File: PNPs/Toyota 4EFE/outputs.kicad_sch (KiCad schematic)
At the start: 9 parts, among them Q2 SSM3K357R, Q3 SSM3K357R, U9 VNLD5090

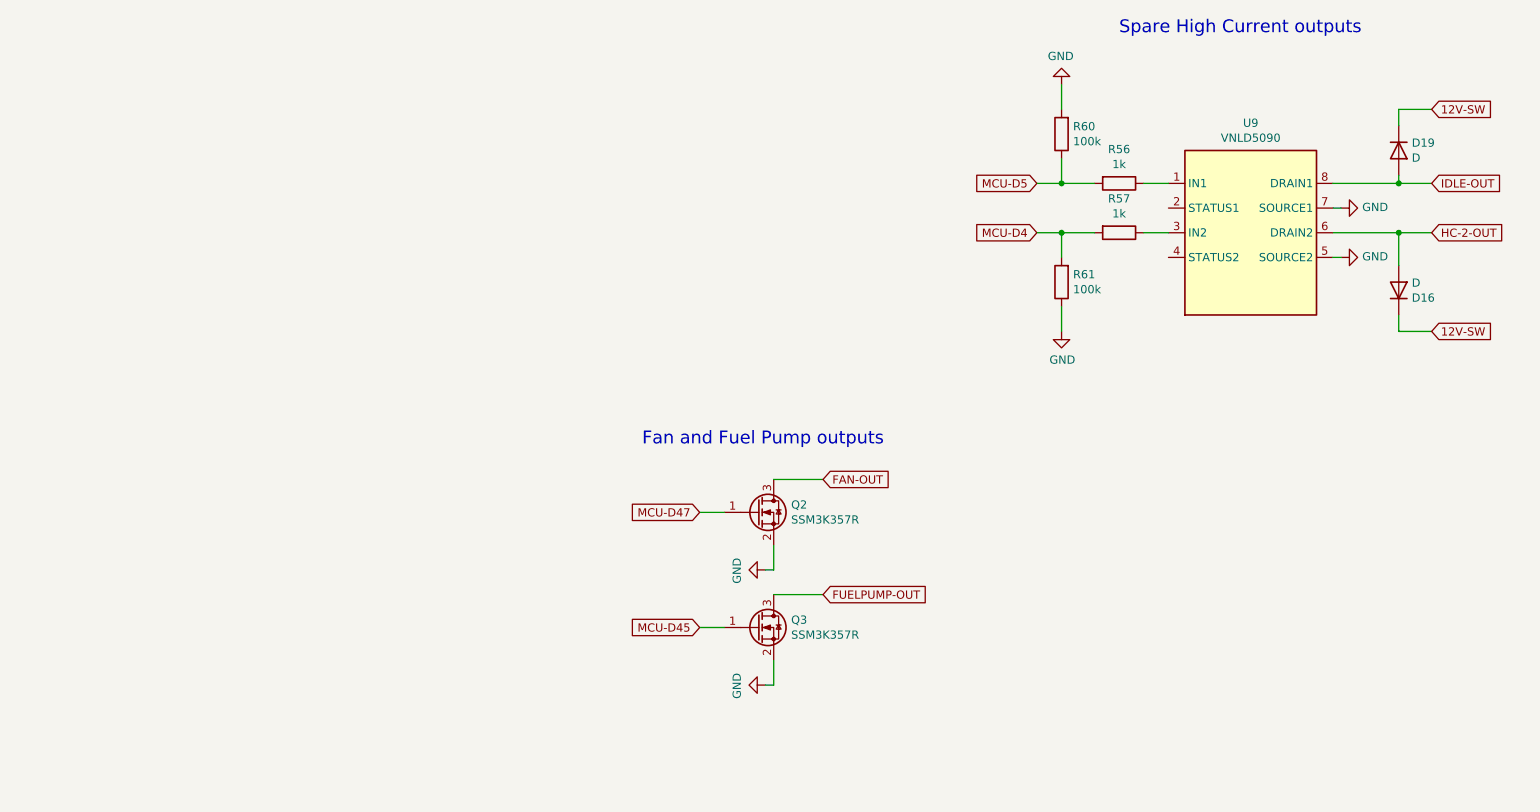
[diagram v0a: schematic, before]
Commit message: Board layout done
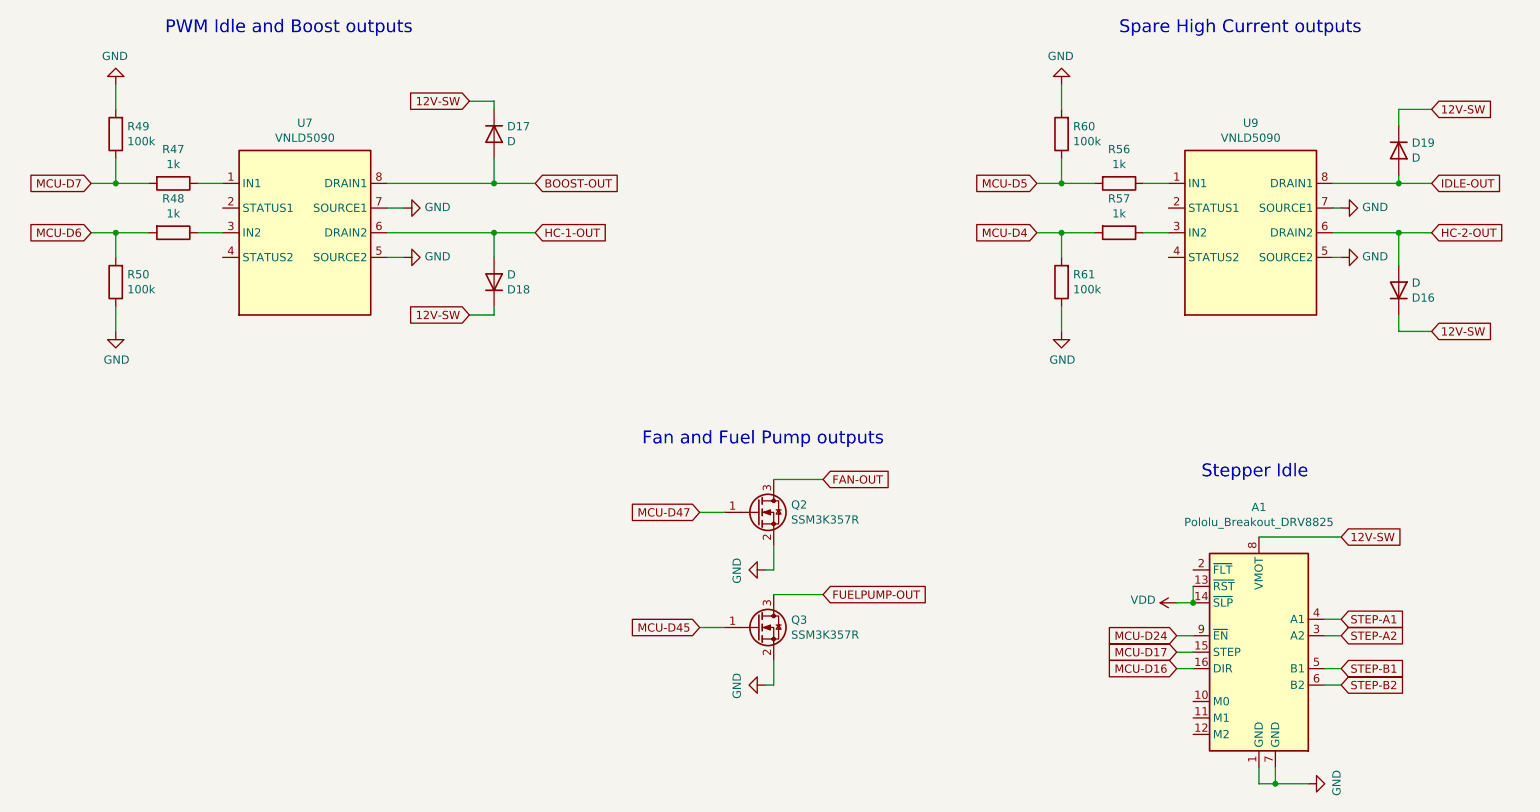
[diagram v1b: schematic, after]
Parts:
- added A1: Pololu_Breakout_DRV8825, Module:Pololu_Breakout-16_15.2x20.3mm, symbol Driver_Motor:Pololu_Breakout_DRV8825
- added D17, D18: D, Diode_SMD:D_SOD-123F, symbol Device:D
- added R47, R48: 1k, Resistor_SMD:R_0805_2012Metric, symbol Device:R
- added R49, R50: 100k, Resistor_SMD:R_0805_2012Metric, symbol Device:R
- added U7: VNLD5090, Package_SO:SOIC-8_3.9x4.9mm_P1.27mm, symbol v0.4.4c-rescue:VNLD5090-IC_Automotive
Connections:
- net 12V-SW: now also A1.8 (VMOT), D17.1 (K), D18.1 (K)
- net GND: now also A1.1 (GND), A1.7 (GND), R49.2, R50.1, U7.5 (SOURCE2), U7.7 (SOURCE1)
- new net: R47.1, U7.1 (IN1)
- new net: R48.1, U7.3 (IN2)
- new net BOOST-OUT: D17.2 (A), U7.8 (DRAIN1)
- new net HC-1-OUT: D18.2 (A), U7.6 (DRAIN2)
- new net MCU-D16: A1.16 (DIR)
- new net MCU-D17: A1.15 (STEP)
- new net MCU-D24: A1.9 (~{EN})
- new net MCU-D6: R48.2, R50.2
- new net MCU-D7: R47.2, R49.1
- new net STEP-A1: A1.4 (A1)
- new net STEP-A2: A1.3 (A2)
- new net STEP-B1: A1.5 (B1)
- new net STEP-B2: A1.6 (B2)
- new net VDD: A1.13 (~{RST}), A1.14 (~{SLP})
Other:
- note added: "PWM Idle and Boost outputs"
- note added: "Stepper Idle"
